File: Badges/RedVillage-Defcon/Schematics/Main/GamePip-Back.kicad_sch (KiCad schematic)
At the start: 52 parts, among them IC1 ESP32-S2-WROOM-I_M22S2H3200US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, J1 2.8" Display, J10 Conn_01x01, J11 Conn_01x01, J13 Conn_02x03_Odd_Even, J2 USB_C_Plug_USB2.0, J3 Conn_01x03, J4 Cap Sense, J5 Cap Sense, J6 Conn_01x05, J7 Conn_01x02, J9 Conn_01x01, Q2 Q_NPN_BCE, SW1 SW_SPDT, SW1 Up, SW2 Down, SW3 Boot, SW3 Left, SW4 A, SW5 Right, SW6 B, SW7 Start/Sel, SW9 RotaryEncoder_Switch, U2 SK6812_Side, U4 SK6812_Side, U5 SK6812_Side, U6 SK6812_Side

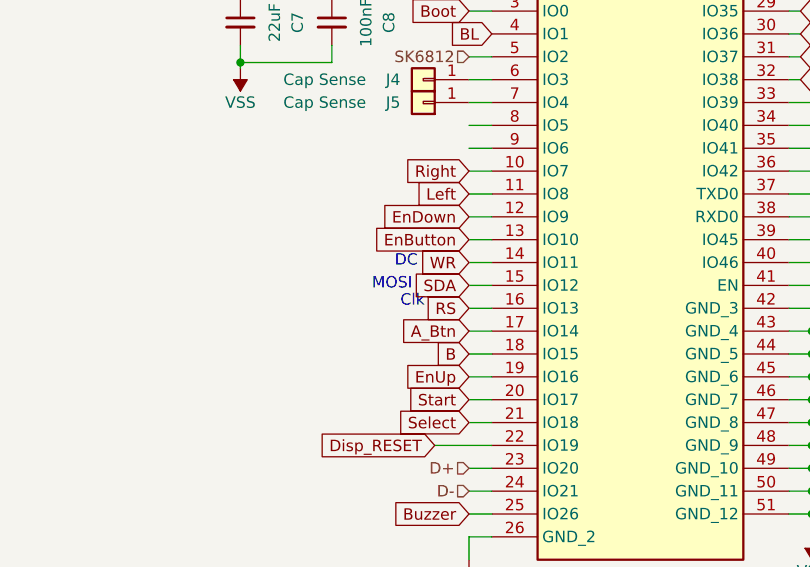
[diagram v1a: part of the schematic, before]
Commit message: Ready to start PCB
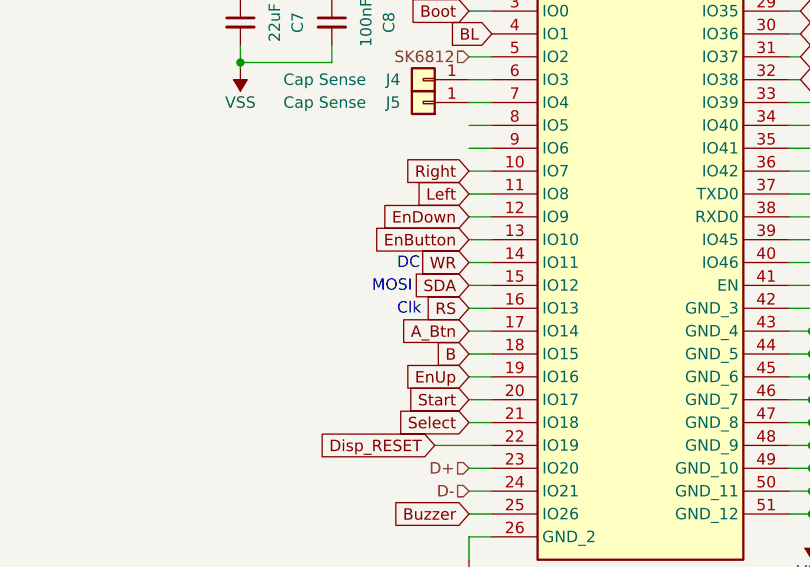
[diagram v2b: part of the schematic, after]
